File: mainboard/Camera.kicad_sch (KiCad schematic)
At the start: 13 parts, among them IC1201 TXB0102DCU, IC1202 PCA9306JK, X1201 Camera, Y1201 25 MHz

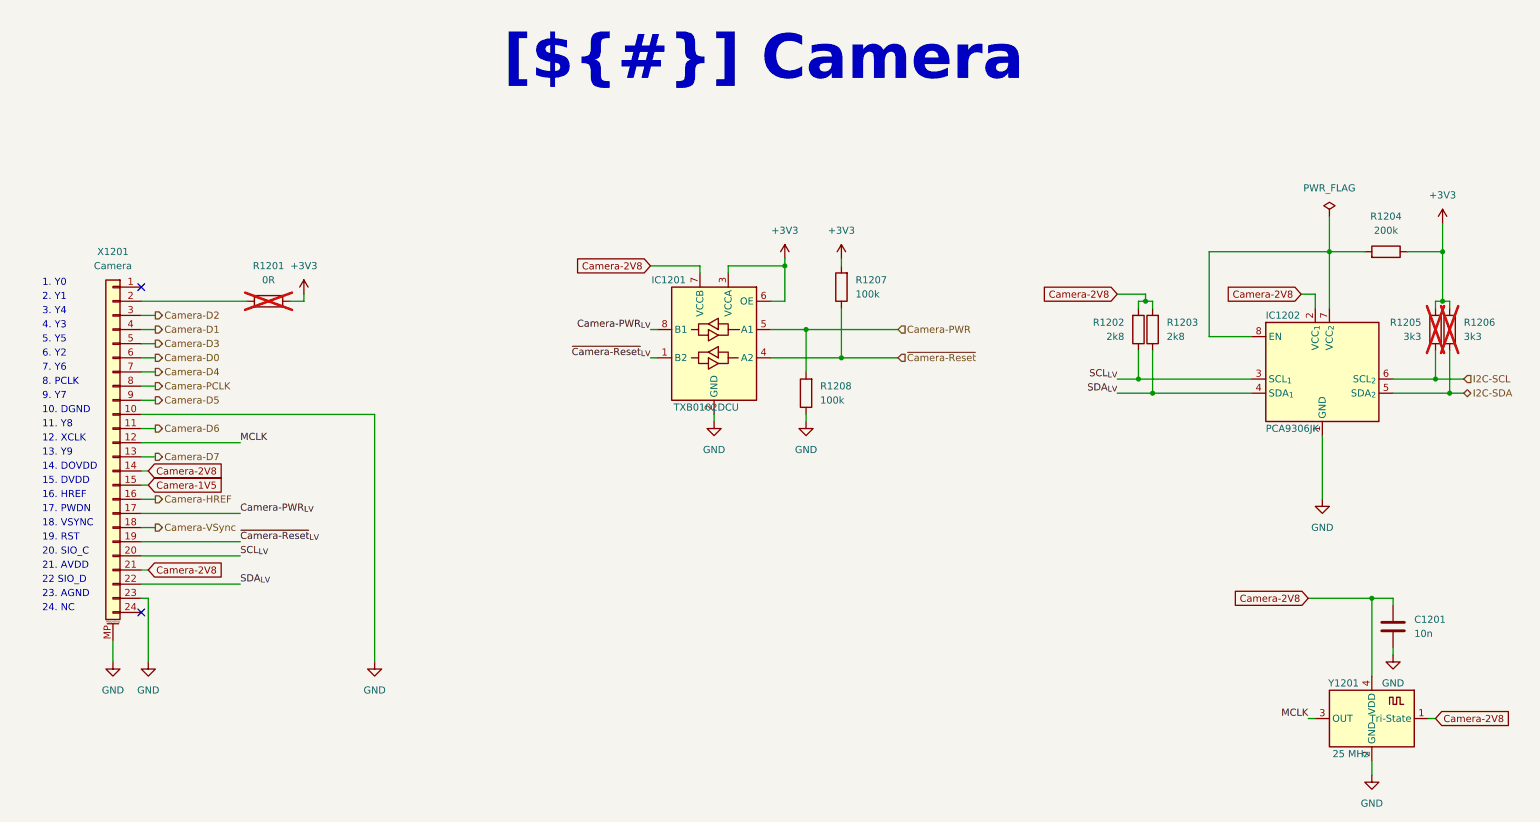
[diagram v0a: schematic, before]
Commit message: Layout complete
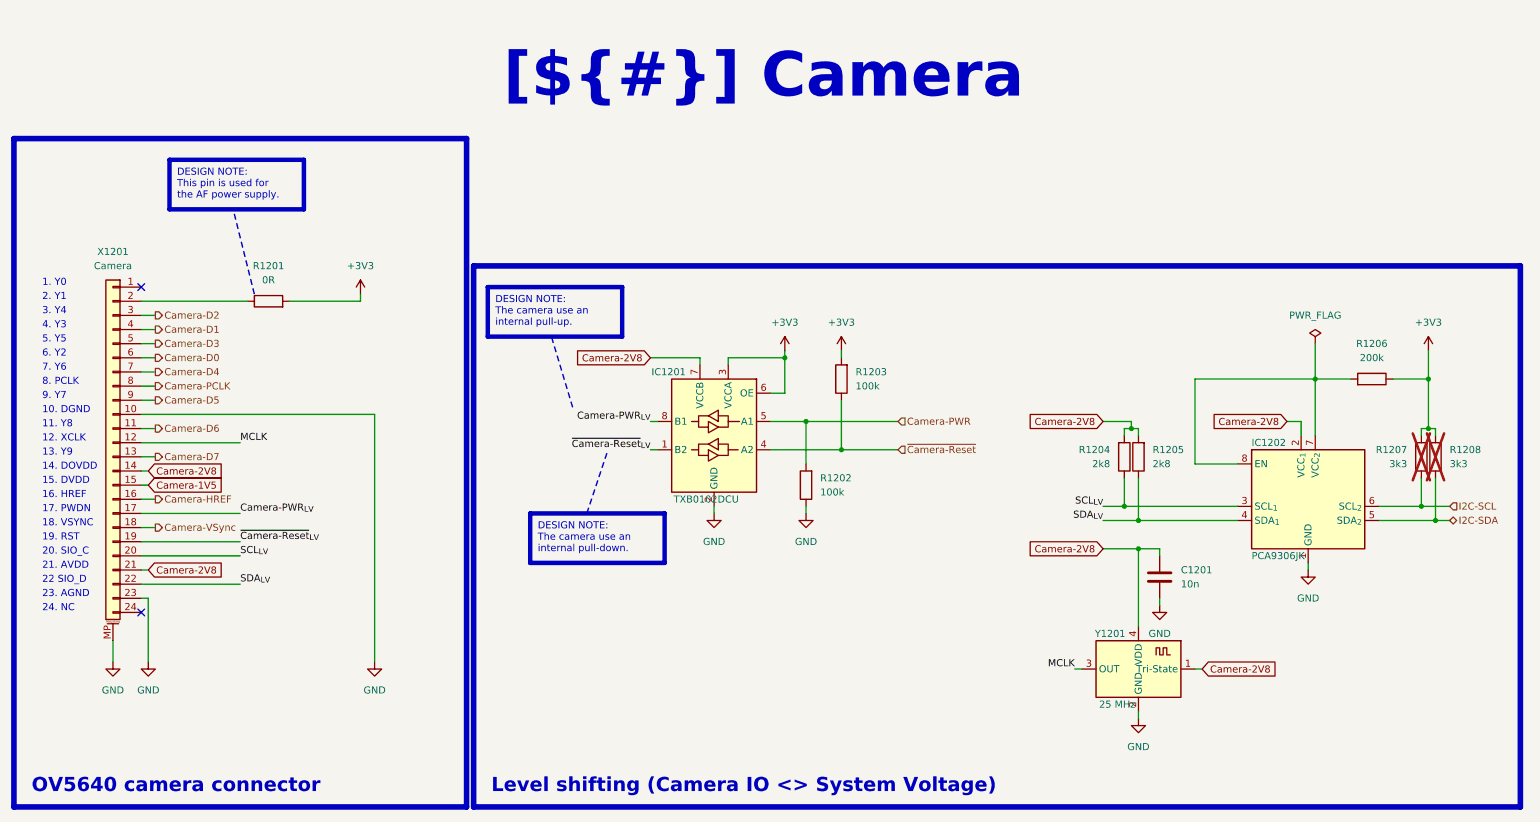
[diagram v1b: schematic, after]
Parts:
- R1201: now fitted
- renumbered R1208 to R1202, R1207 to R1203, R1202 to R1204, R1203 to R1205, R1204 to R1206, R1205 to R1207, R1206 to R1208
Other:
- moved on the sheet: C1201, IC1201, IC1202, R1202, R1203, R1204, R1205, R1206, R1207, R1208, Y1201
